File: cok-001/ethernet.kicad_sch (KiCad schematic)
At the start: 59 parts, among them J3501 RJ45, U3501 BD3520FVM-TR, U3502 MM1761KHBE, U3503 88E6108, Y3501 25MHz

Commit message: msop
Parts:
- U3501: footprint Package_SO:MSOP-8_3x3mm_P0.65mm -> PS3:MSOP-8_2.9x4mm_P0.65mm
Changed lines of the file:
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@@
 			)
 		)
-		(property "Footprint" "Package_SO:MSOP-8_3x3mm_P0.65mm"
+		(property "Footprint" "PS3:MSOP-8_2.9x4mm_P0.65mm"
 			(at 96.52 210.82 0)
 			(effects

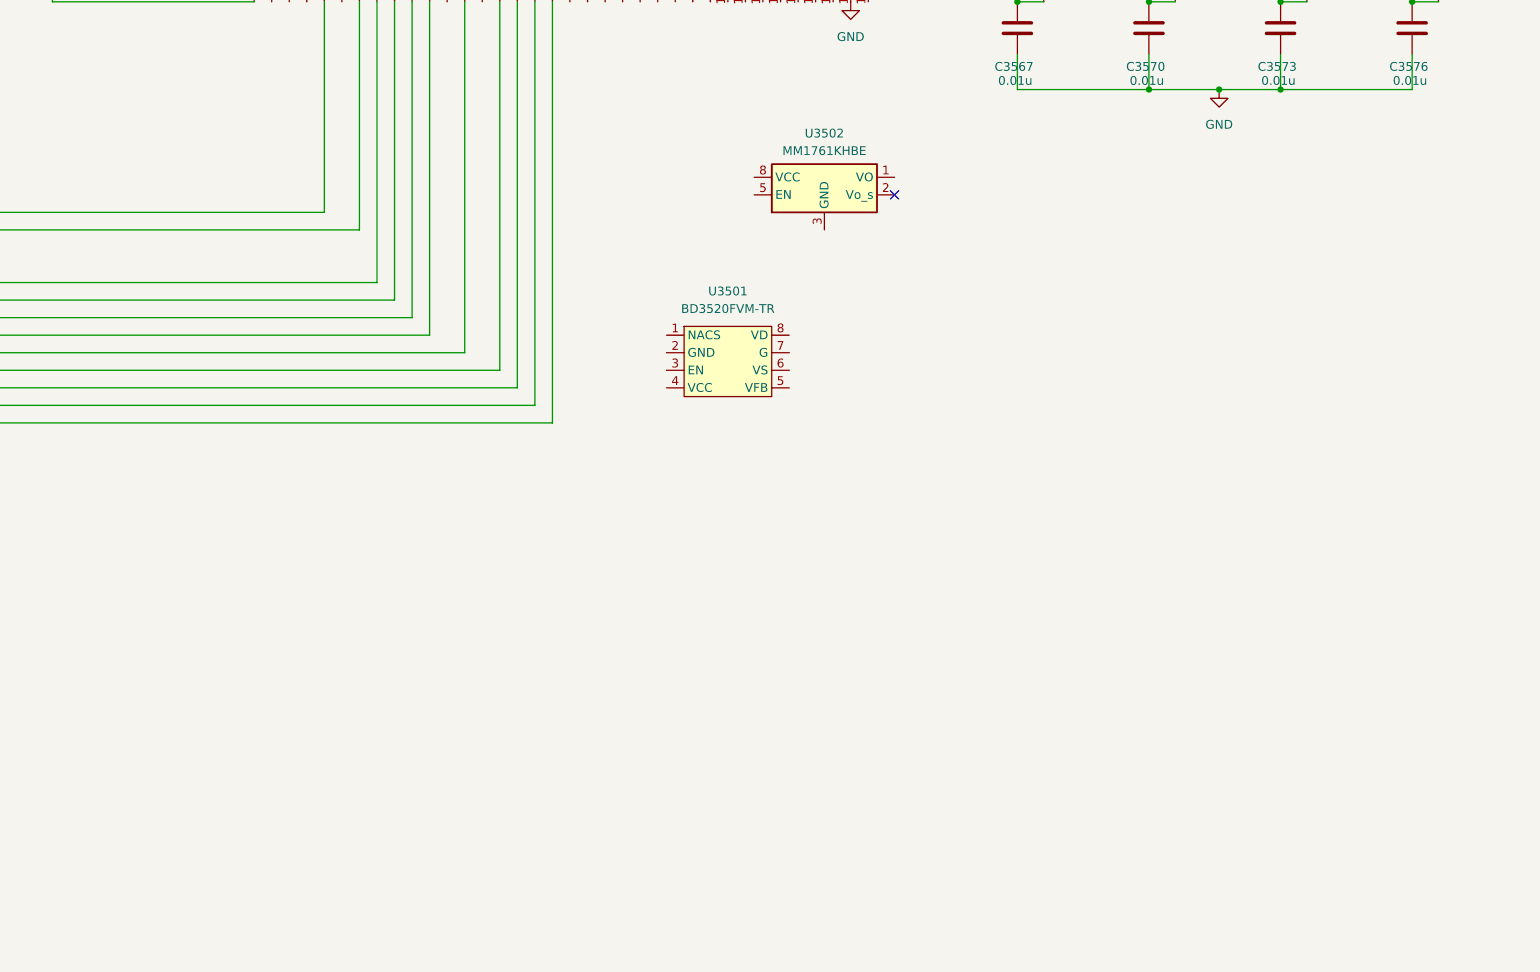
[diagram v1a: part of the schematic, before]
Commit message: voltage symbols
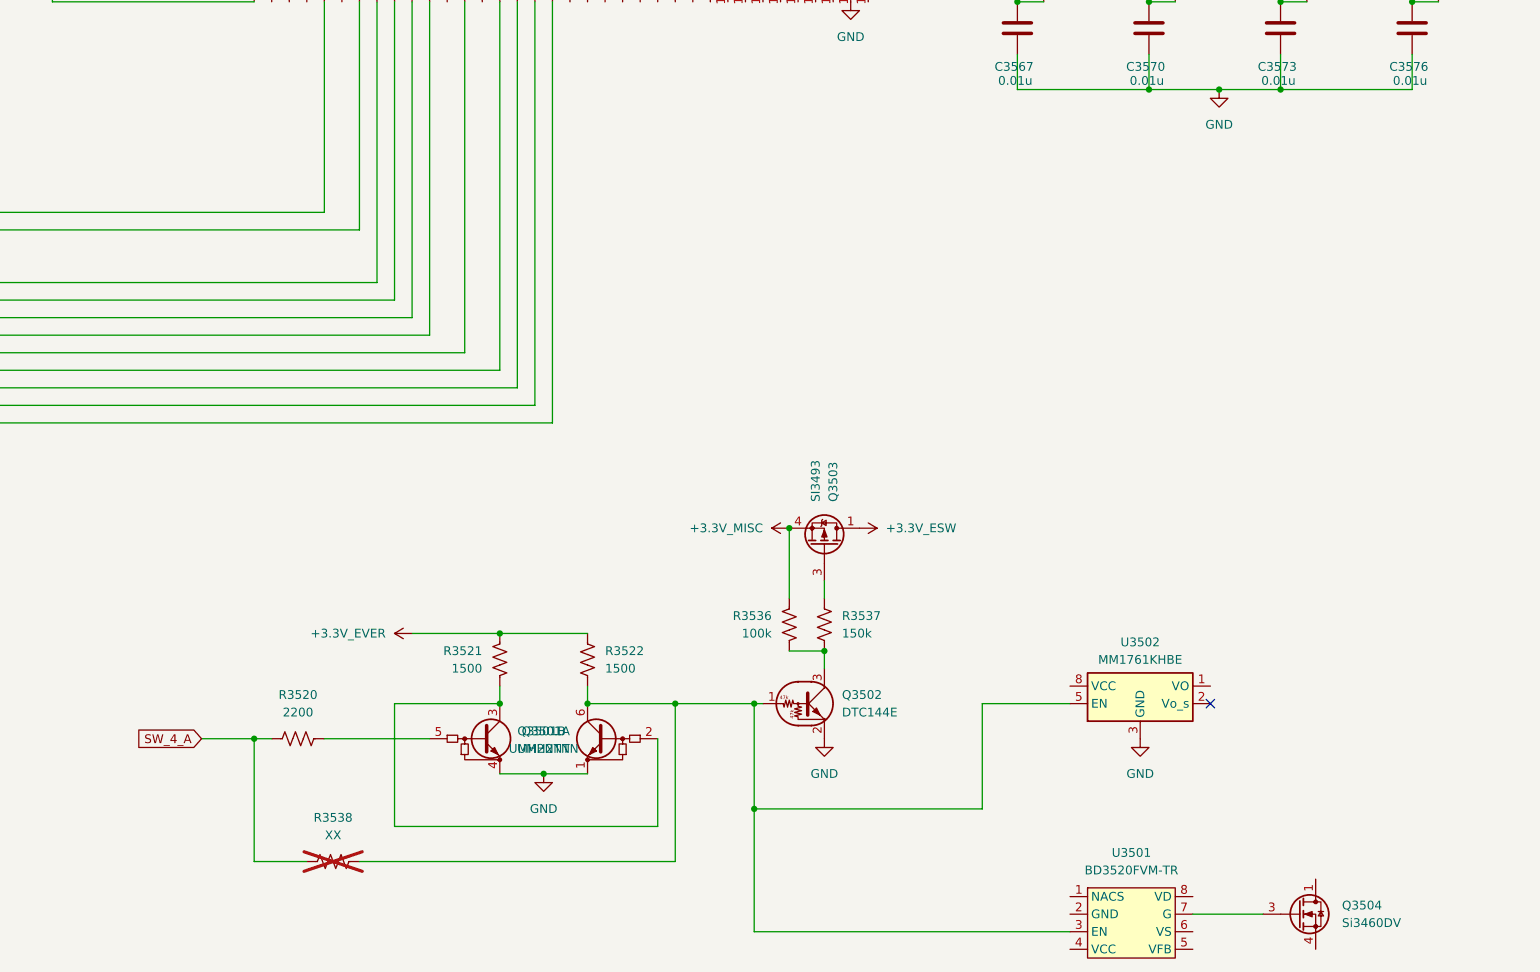
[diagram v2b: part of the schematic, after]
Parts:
- added Q3501: UMH2NTN, Package_TO_SOT_SMD:SOT-363_SC-70-6, symbol Transistor_BJT:MUN5213DW1
- added Q3502: DTC144E, Package_TO_SOT_SMD:SOT-323_SC-70, symbol Transistor_BJT:DTC144E
- added Q3503: SI3493, Package_SO:TSOP-6_1.65x3.05mm_P0.95mm, symbol Transistor_FET:PMN48XP
- added Q3504: Si3460DV, Package_SO:TSOP-6_1.65x3.05mm_P0.95mm, symbol Transistor_FET:Si3456DDV
- added R3520: 2200, Resistor_SMD:R_0402_1005Metric, symbol Device:R_US
- added R3521, R3522: 1500, Resistor_SMD:R_0402_1005Metric, symbol Device:R_US
- added R3536: 100k, Resistor_SMD:R_0402_1005Metric, symbol Device:R_US
- added R3537: 150k, Resistor_SMD:R_0402_1005Metric, symbol Device:R_US
- added R3538: XX, Resistor_SMD:R_0402_1005Metric, symbol Device:R_US
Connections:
- net GND: now also U3502.3 (GND), U3502.4 (GND), U3502.6 (GND), U3502.7 (GND), U3502.9 (GND), Q3501.1 (E1), Q3501.4 (E2), Q3502.2 (E)
- net at U3502.5 (EN): now also U3501.3 (EN), Q3501.6 (C1), Q3502.1 (B), R3522.1, R3538.2
- net at U3501.7 (G): now also Q3504.3 (G)
- new net: Q3502.3 (C), R3536.1, R3537.1
- new net: Q3503.3 (G), R3537.2
- new net: Q3501.5 (B2), R3520.2
- new net: Q3504.1 (D), Q3504.2 (D), Q3504.5 (D), Q3504.6 (D)
- new net: Q3501.2 (B1), Q3501.3 (C2), R3521.1
- new net +3.3V_ESW: Q3503.1 (D), Q3503.2 (D), Q3503.5 (D), Q3503.6 (D)
- new net +3.3V_EVER: R3521.2, R3522.2
- new net +3.3V_MISC: Q3503.4 (S), R3536.2
- new net SW_4_A: R3520.1, R3538.1
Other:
- moved on the sheet: U3501, U3502
